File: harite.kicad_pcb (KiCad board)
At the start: 2 copper layers, 153.5 x 121.8 mm, 39 parts, among them U1 RP2040_Zero

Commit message: Fix usb
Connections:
- USB1 pad 11: unconnected-(USB1-VBUS-Pad11) -> 5V
- USB1 pad 6: GP0 -> GP1
- USB1 pad 7: GP1 -> GP0
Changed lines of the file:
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@@
 	(net 67 "SO")
 	(net 68 "unconnected-(USB1-CC1-Pad4)")
-	(net 69 "unconnected-(USB1-VBUS-Pad11)")
-	(net 70 "unconnected-(USB1-CC2-Pad10)")
-	(net 71 "unconnected-(USB1-SBU1-Pad9)")
-	(net 72 "unconnected-(USB1-SBU2-Pad3)")
+	(net 69 "unconnected-(USB1-CC2-Pad10)")
+	(net 70 "unconnected-(USB1-SBU1-Pad9)")
+	(net 71 "unconnected-(USB1-SBU2-Pad3)")
 	(footprint "ScottoKeebs_Components:Diode_SOD-123"
 		(layer "F.Cu")
@@
 			(size 0.3 1.45)
 			(layers "F.Cu" "F.Paste" "F.Mask")
-			(net 72 "unconnected-(USB1-SBU2-Pad3)")
+			(net 71 "unconnected-(USB1-SBU2-Pad3)")
 			(pinfunction "SBU2")
 			(pintype "input")
@@
 			(size 0.3 1.45)
 			(layers "F.Cu" "F.Paste" "F.Mask")
-			(net 48 "GP0")
+			(net 50 "GP1")
 			(pinfunction "DP1")
 			(pintype "input")
@@
 			(size 0.3 1.45)
 			(layers "F.Cu" "F.Paste" "F.Mask")
-			(net 50 "GP1")
+			(net 48 "GP0")
 			(pinfunction "DN1")
 			(pintype "input")
@@
 			(size 0.3 1.45)
 			(layers "F.Cu" "F.Paste" "F.Mask")
-			(net 71 "unconnected-(USB1-SBU1-Pad9)")
+			(net 70 "unconnected-(USB1-SBU1-Pad9)")
 			(pinfunction "SBU1")
 			(pintype "input")
@@
 			(size 0.3 1.45)
 			(layers "F.Cu" "F.Paste" "F.Mask")
-			(net 70 "unconnected-(USB1-CC2-Pad10)")
+			(net 69 "unconnected-(USB1-CC2-Pad10)")
 			(pinfunction "CC2")
 			(pintype "input")
@@
 			(size 0.6 1.45)
 			(layers "F.Cu" "F.Paste" "F.Mask")
-			(net 69 "unconnected-(USB1-VBUS-Pad11)")
+			(net 52 "5V")
 			(pinfunction "VBUS")
 			(pintype "input")

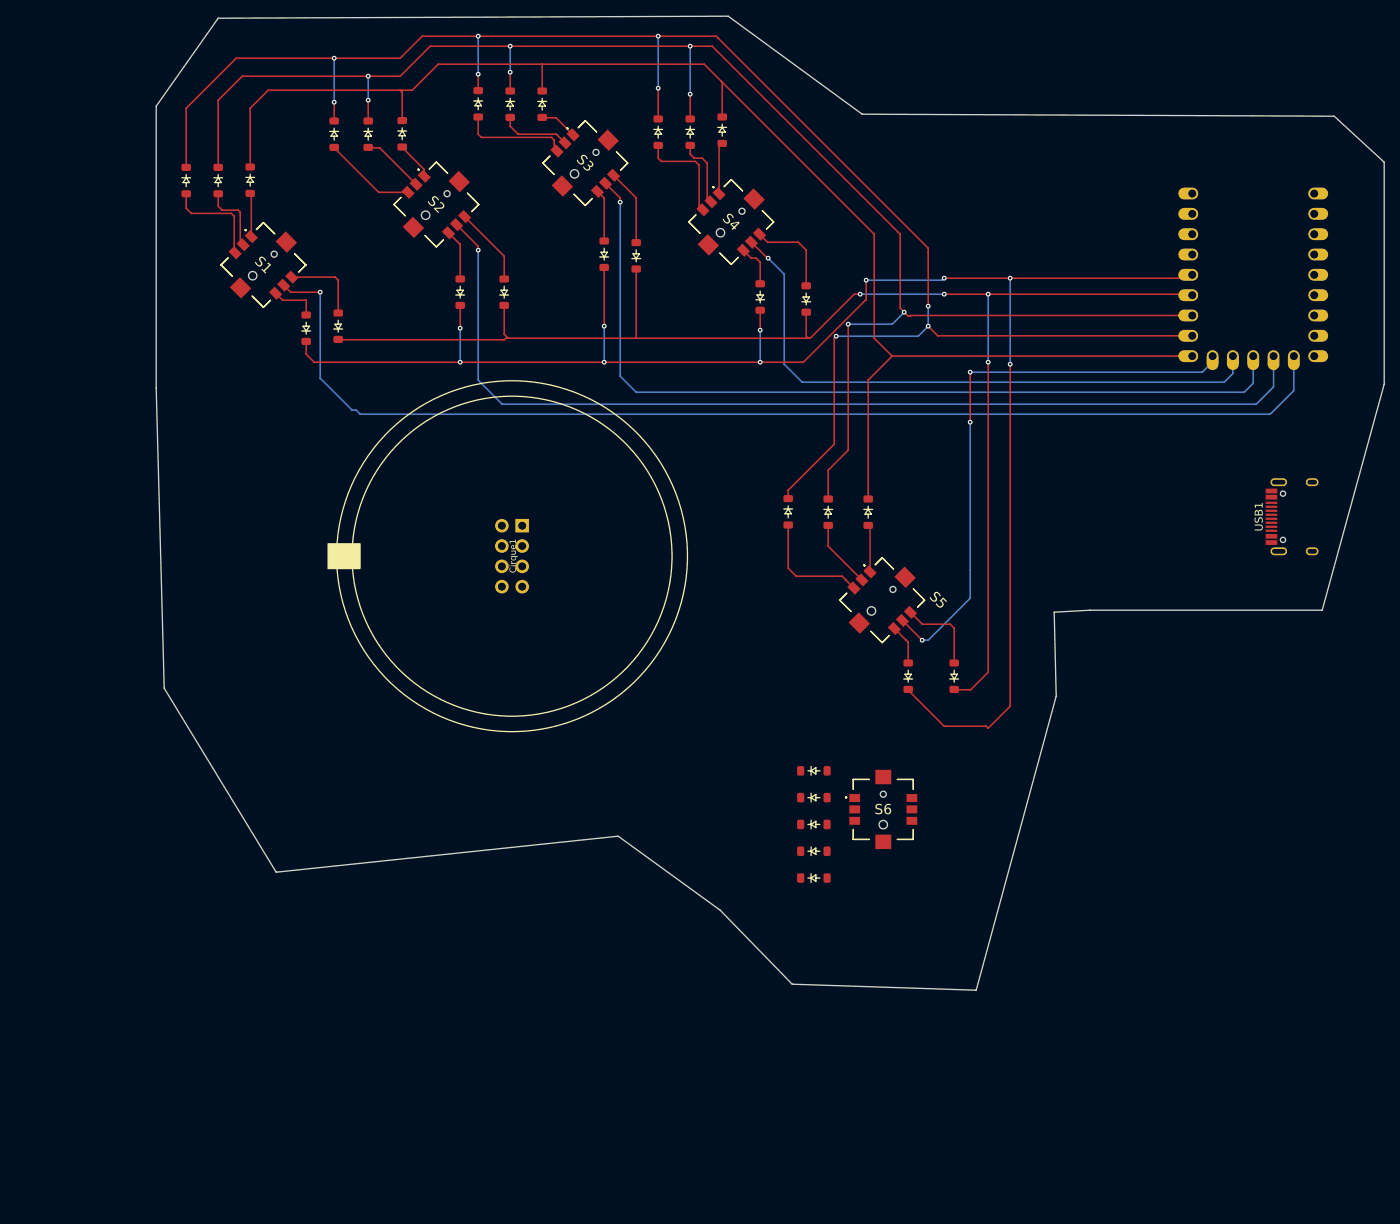
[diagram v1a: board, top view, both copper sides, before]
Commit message: Shaping
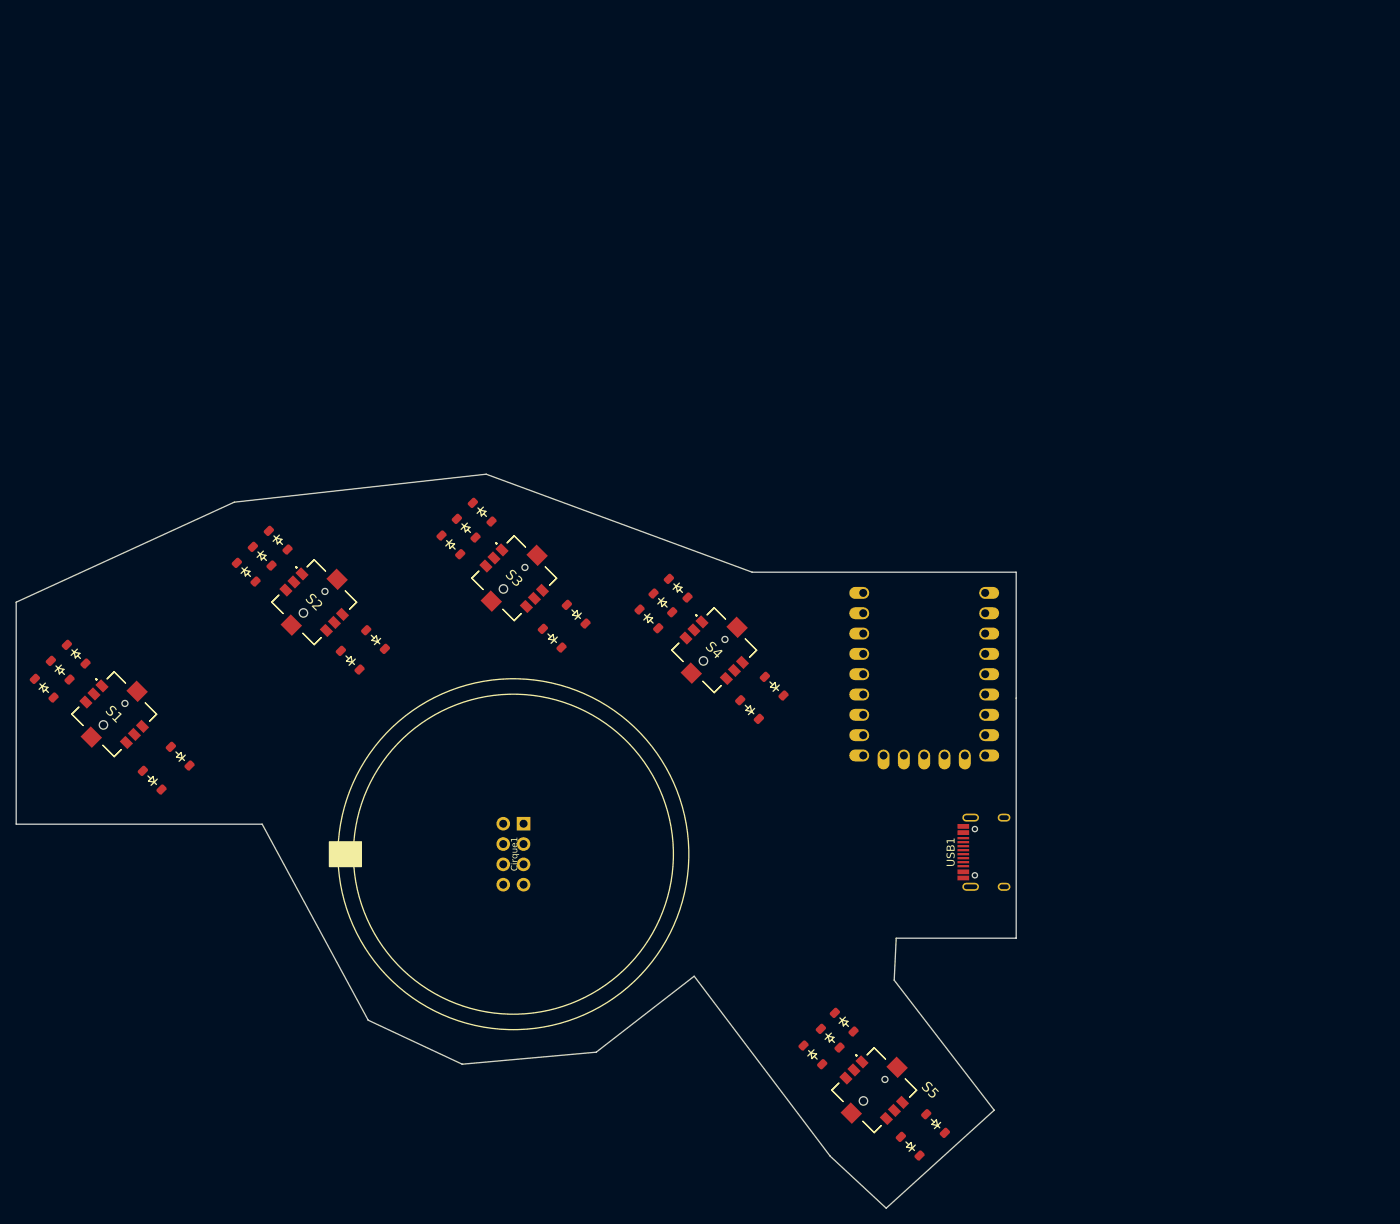
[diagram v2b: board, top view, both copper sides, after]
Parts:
- removed D26, D27, D28, D29, D30: D, ScottoKeebs_Components:Diode_SOD-123
- removed S6: SKRHADE010, footprints:SKRHADE010
- moved D5 75.4 mm to (104.8, 108.2), turned to 135 degrees
- moved D23 68.0 mm to (187.3, 142.6), turned to -45 degrees
- moved D22 65.8 mm to (189.5, 140.5), turned to -45 degrees
- moved U1 64.7 mm to (201.2, 95.0)
- moved D21 63.8 mm to (191.2, 138.5), turned to -45 degrees
- moved D2 63.2 mm to (93.2, 94.5), turned to -45 degrees
- moved D1 63.1 mm to (95.2, 92.5), turned to -45 degrees
- moved S5 61.3 mm to (195.0, 147.0)
- moved D18 60.8 mm to (166.8, 88.1), turned to -45 degrees
- moved S1 59.2 mm to (100.0, 100.0)
- moved D17 58.9 mm to (168.6, 86.1), turned to -45 degrees
- moved D25 58.8 mm to (199.5, 154.0), turned to 135 degrees
- moved D16 57.5 mm to (170.5, 84.2), turned to -45 degrees
- moved D4 57.3 mm to (108.2, 105.2), turned to 135 degrees
- moved USB1 56.9 mm to (213.8, 117.2)
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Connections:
- U1 pad 10: Col 2 -> Col 1
- U1 pad 11: Col 3 -> Col 2
- U1 pad 12: Col 4 -> Col 3
- U1 pad 13: Col 5 -> Col 4
- U1 pad 14: Col 6 -> Col 5
- U1 pad 9: Col 1 -> unconnected-(U1-8-Pad9)
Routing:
- net Row 2: track 217.7 -> 0.00 mm, vias 9 -> 0
- net Row 5: track 213.4 -> 0.00 mm, vias 10 -> 0
- net Row 3: track 202.9 -> 0.00 mm, vias 8 -> 0
- net Row 1: track 180.7 -> 0.00 mm
- net Row 4: track 177.8 -> 0.00 mm, vias 4 -> 0
- net Col 1: track 144.8 -> 0.00 mm, vias 1 -> 0
- net Col 2: track 126.0 -> 0.00 mm, vias 1 -> 0
- net Col 3: track 108.7 -> 0.00 mm, vias 1 -> 0
- net Col 4: track 76.6 -> 0.00 mm, vias 1 -> 0
- net Col 5: track 71.5 -> 0.00 mm, vias 3 -> 0
- net Net-(D23-A): track 14.6 -> 0.00 mm
- net Net-(D13-A): track 13.4 -> 0.00 mm
- net Net-(D18-A): track 12.8 -> 0.00 mm
- net Net-(D2-A): track 12.8 -> 0.00 mm
- net Net-(D8-A): track 11.5 -> 0.00 mm
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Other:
- board size 153.5 x 121.8 mm -> 125 x 91.8 mm
